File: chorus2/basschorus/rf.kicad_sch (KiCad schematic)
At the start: 11 parts, among them U4 TL074

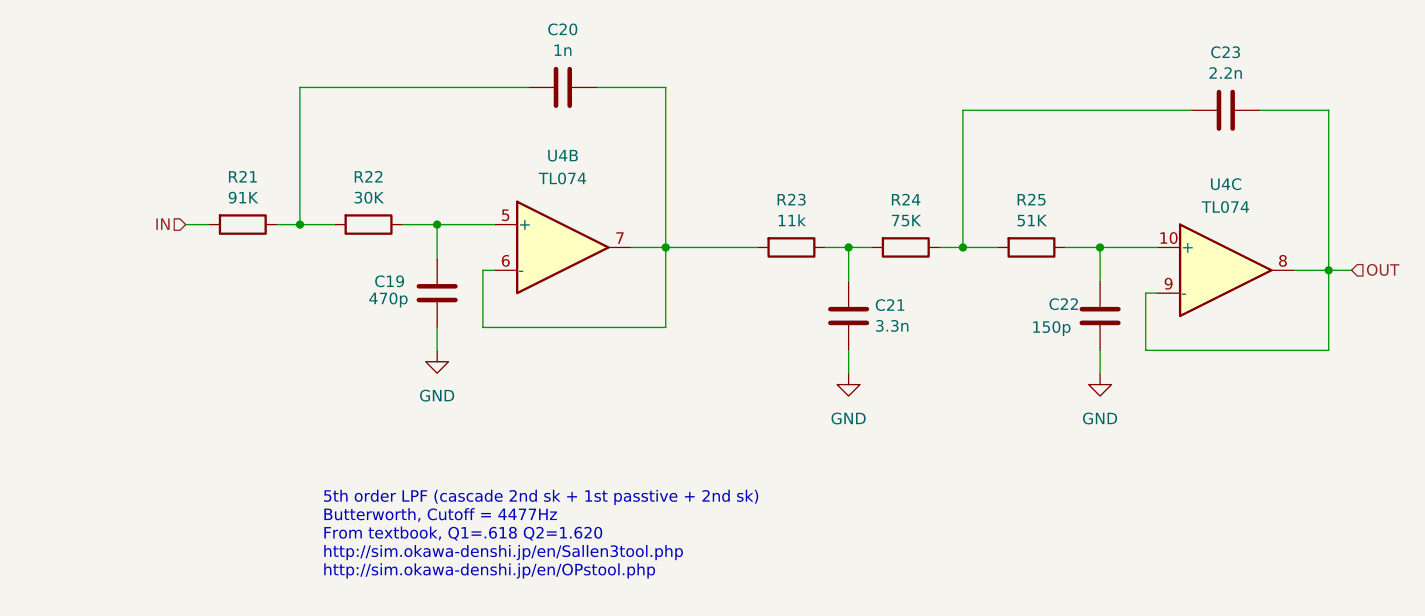
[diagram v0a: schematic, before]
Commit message: update filters
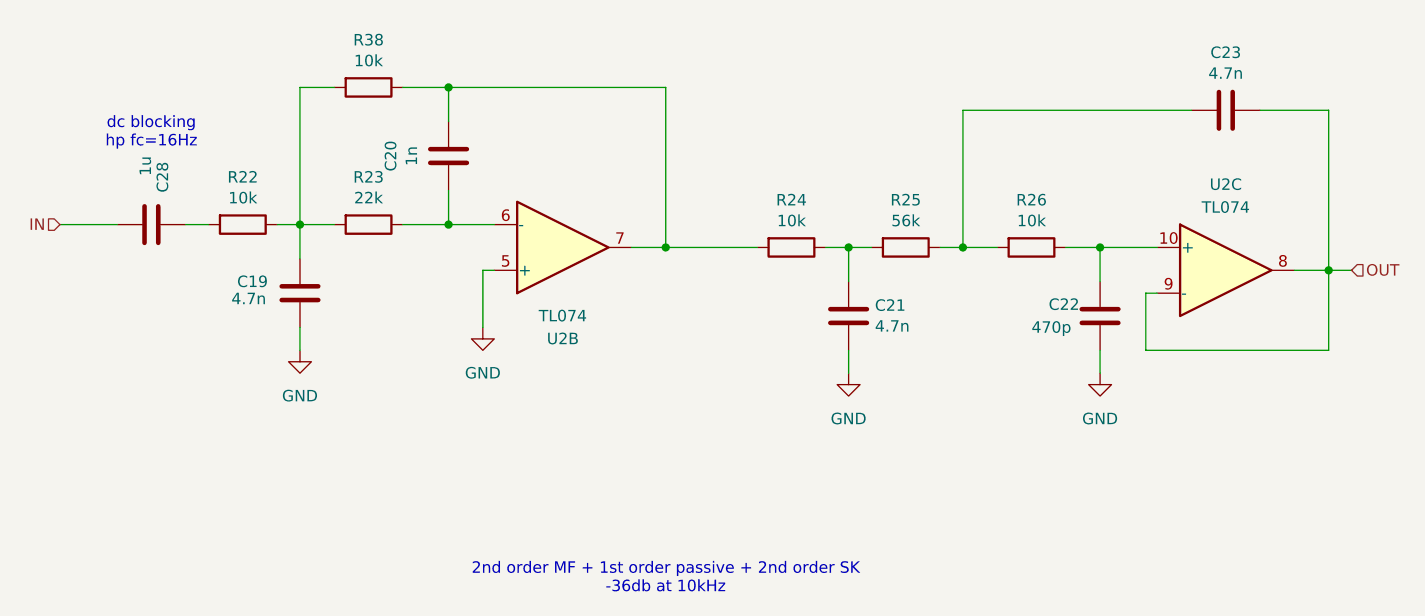
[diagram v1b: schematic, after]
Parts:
- added C28: 1u, symbol Device:C
- added R38: 10k, kicad-legacy/kicad-footprints/Resistor_THT.pretty:R_Axial_DIN0204_L3.6mm_D1.6mm_P2.54mm_Vertical, symbol Device:R
- C19: value 470p -> 4.7n
- C21: value 3.3n -> 4.7n
- C22: value 150p -> 470p
- C23: value 2.2n -> 4.7n
- R22: renamed from R21; value 91K -> 10k
- R23: renamed from R22; value 30K -> 22k
- R24: renamed from R23; value 11k -> 10k
- R25: renamed from R24; value 75K -> 56k
- R26: renamed from R25; value 51K -> 10k
- renumbered U4 to U2
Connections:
- net GND: now also U2.5 (+)
- net IN: now also C28.1; no longer R22.2
- net at R22.1, R23.2: now also C19.2, R38.2; no longer C20.2
- net at C20.1, R24.2, U2.7: now also R38.1; no longer U2.6 (-)
- new net: C20.2, R23.1, U2.6 (-)
- new net: C28.2, R22.2
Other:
- note added: "2nd order MF + 1st order passive + 2nd order SK -36db at 10kHz"
- note added: "dc blocking hp fc=16Hz"
- note removed: "5th order LPF (cascade 2nd sk + 1st passtive + 2nd sk) Butterworth, Cutoff = 4477Hz From textbook, Q1=.618 Q2=1.620 http://sim.okawa-denshi.jp/en/Sallen3tool.php http://sim.okawa-denshi.jp/en/OPstool.php"
- moved on the sheet: C19, C20
